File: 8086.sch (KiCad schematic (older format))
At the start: 1 part

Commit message: sfds
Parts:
- removed U?: 8086_Max_Mode, Package_DIP:DIP-40_W15.24mm, symbol MCU_Intel:8086_Max_Mode
- added U?: 8086_Min_Mode, Package_DIP:DIP-40_W15.24mm, symbol MCU_Intel:8086_Min_Mode
- added U? (x3): 74LS373, symbol 74xx:74LS373
- added U?: 74LS244, symbol 74xx:74LS244
- added U? (x2): 74LS245, symbol 74xx:74LS245
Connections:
- net labels added: GND, VCC
- wire segments 0 -> 124

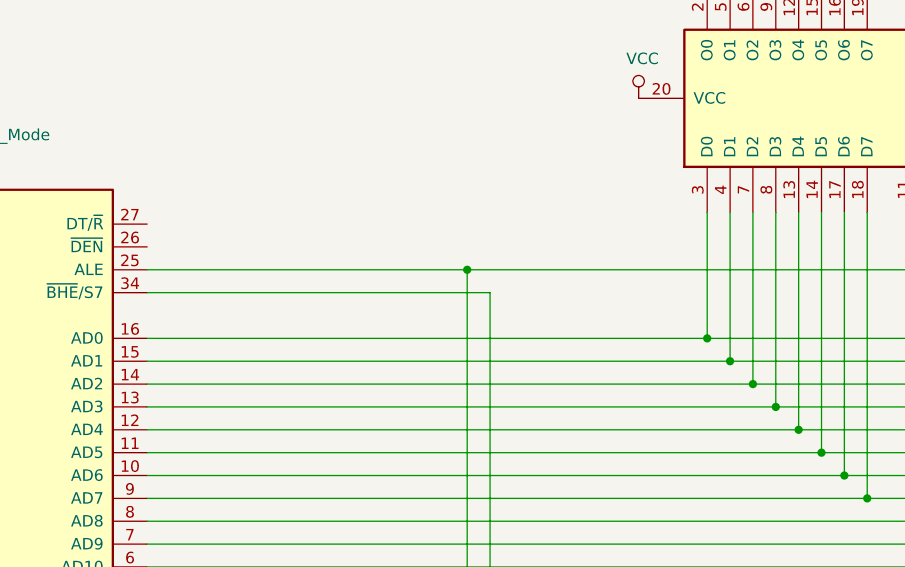
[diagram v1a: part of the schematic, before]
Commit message: 16550 v1
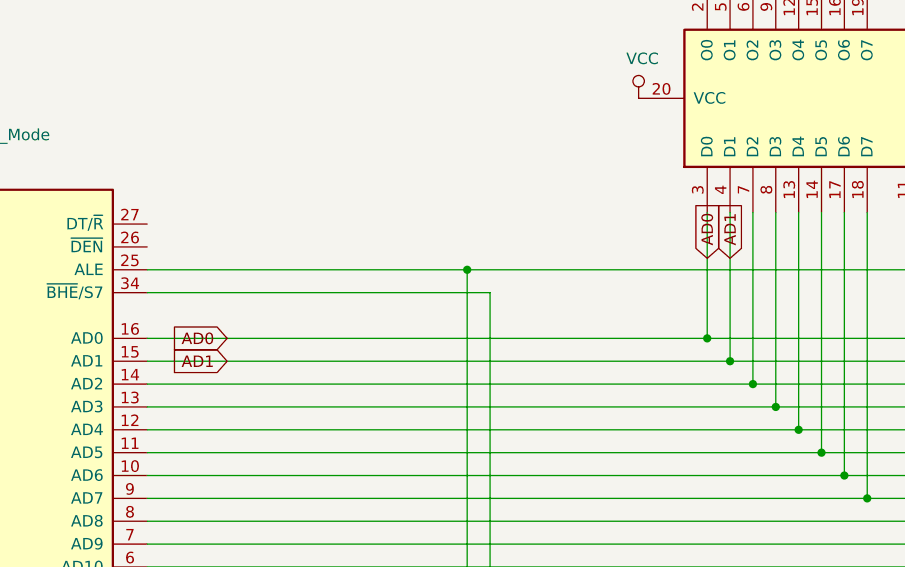
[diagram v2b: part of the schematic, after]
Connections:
- net labels added: AD0, AD1
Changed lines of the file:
@@
 $Descr A4 11693 8268
 encoding utf-8
-Sheet 3 5
+Sheet 3 7
 Title ""
 Date ""
@@
 	0    -1   -1   0
 $EndComp
-Wire Wire Line
-	5300 2850 8700 2850
 $Comp
 L power:GND #PWR?
@@
 	8900 3050 8900 2800
 Wire Wire Line
-	8800 2950 8800 2700
-Wire Wire Line
 	8700 2850 8700 2600
 Wire Wire Line
@@
 Connection ~ 5600 3150
 Connection ~ 5700 3250
-Connection ~ 5300 2850
 Connection ~ 5800 3350
 Wire Wire Line
 	5300 2300 5300 2850
-Wire Wire Line
-	5400 2300 5400 2950
 Wire Wire Line
 	5500 2300 5500 3050
@@
 	1    0    0    -1
 $EndComp
+Text GLabel 3200 2850 0    50   Input ~ 0
+AD0
+Text GLabel 3200 2950 0    50   Input ~ 0
+AD1
+Text GLabel 5400 2500 1    50   Input ~ 0
+AD1
+Text GLabel 5300 2500 1    50   Input ~ 0
+AD0
+Connection ~ 5300 2850
+Wire Wire Line
+	8800 2950 8800 2700
+Wire Wire Line
+	5400 2300 5400 2950
+Wire Wire Line
+	5300 2850 8700 2850
 $EndSCHEMATC

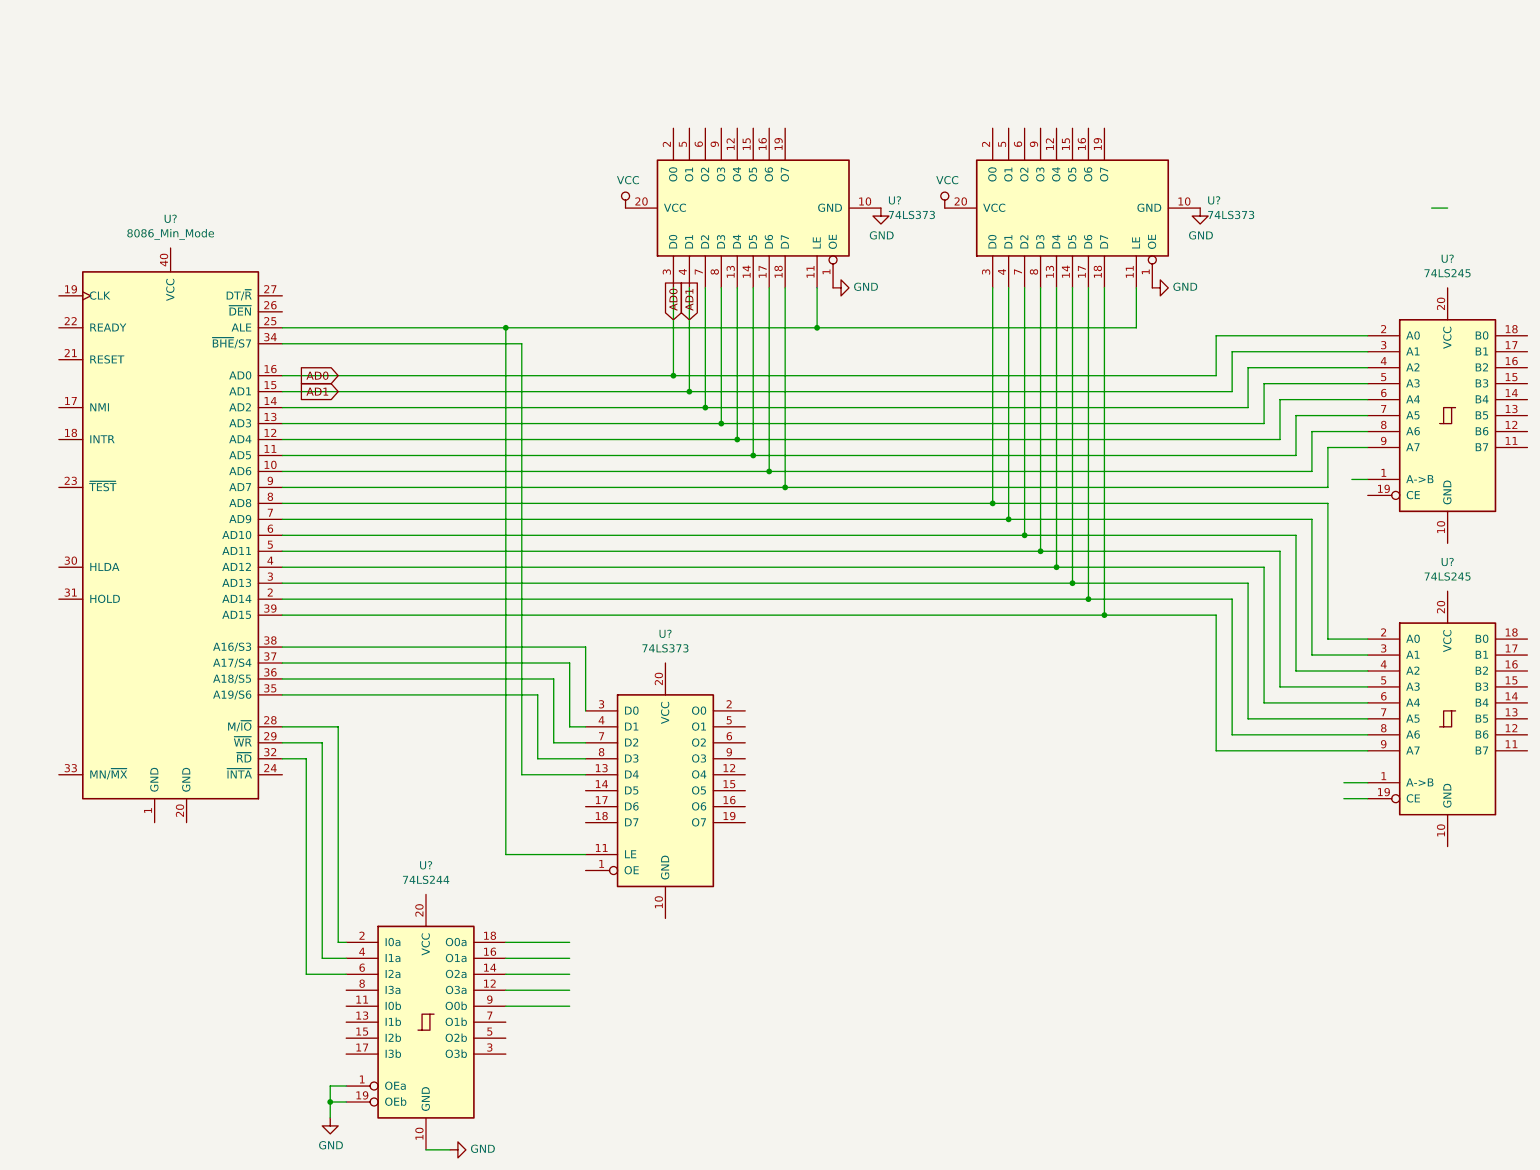
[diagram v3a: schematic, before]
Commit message: update
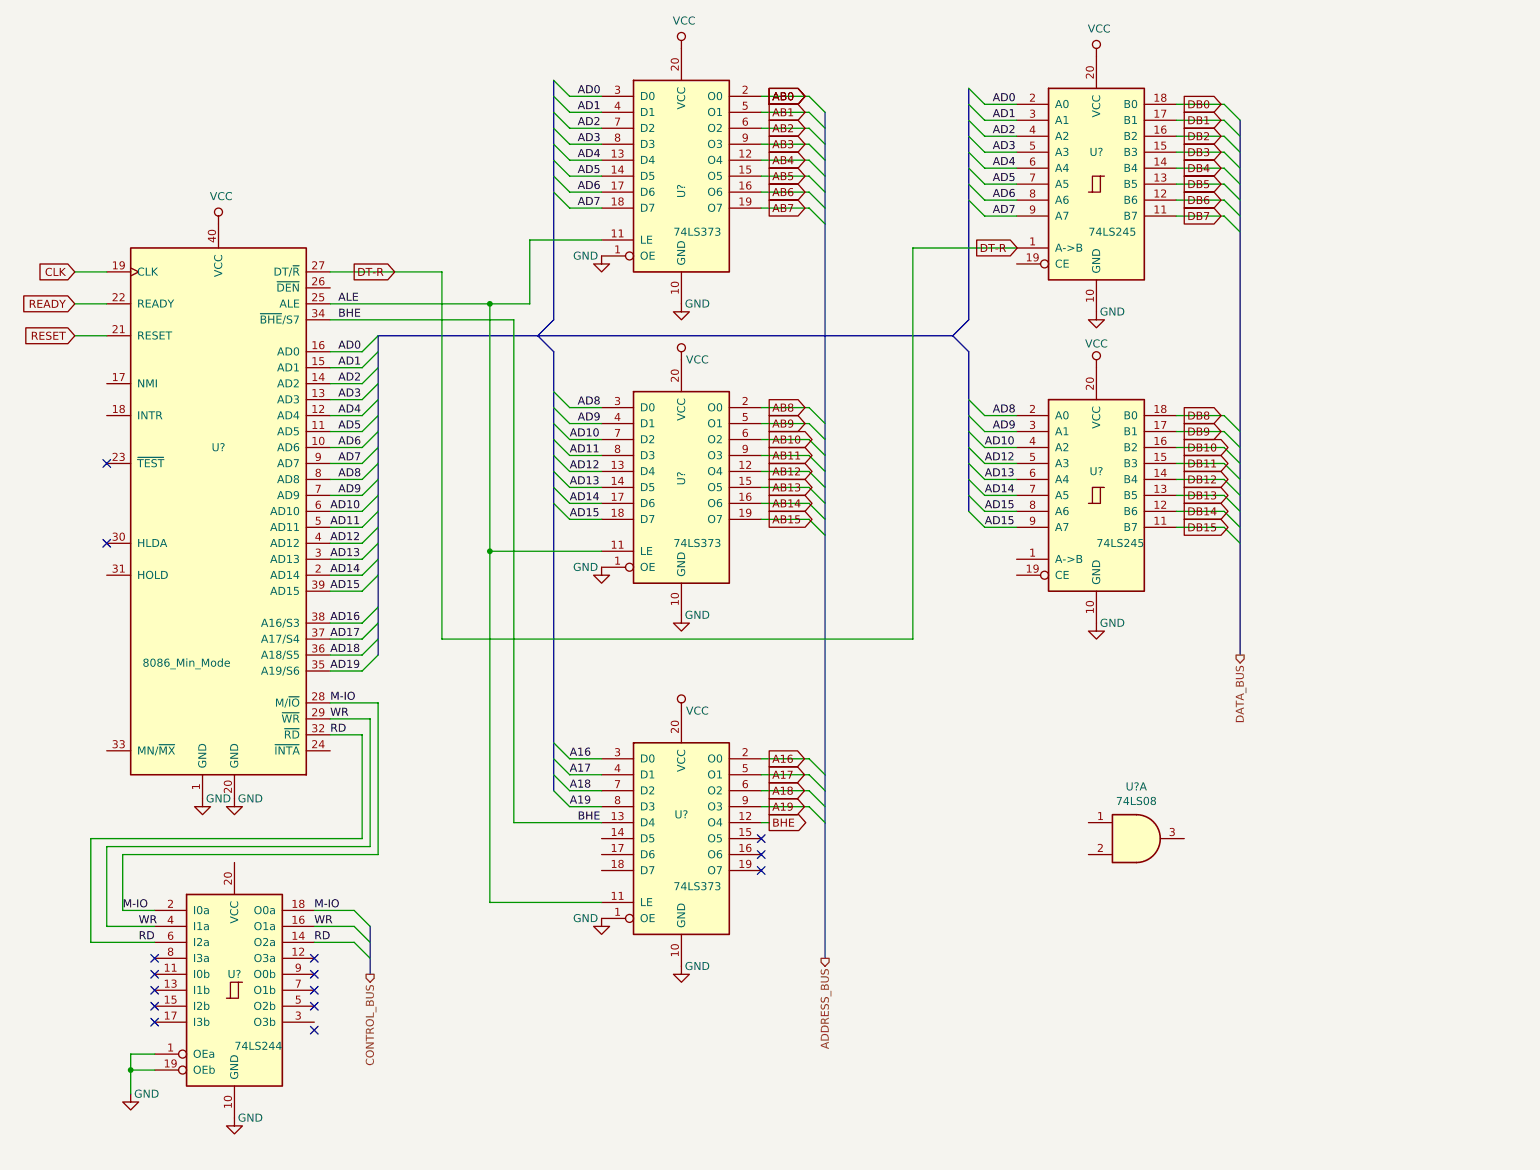
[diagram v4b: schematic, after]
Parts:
- removed U?: 8086_Min_Mode, Package_DIP:DIP-40_W15.24mm, symbol MCU_Intel:8086_Min_Mode
- removed U? (x3): 74LS373, symbol 74xx:74LS373
- removed U?: 74LS244, symbol 74xx:74LS244
- removed U? (x2): 74LS245, symbol 74xx:74LS245
- added U? (x2): 74LS245, symbol 74xx:74LS245
- added U?: 74LS244, symbol 74xx:74LS244
- added U? (x3): 74LS373, symbol 74xx:74LS373
- added U?: 74LS08, symbol 74xx:74LS08
- added U?: 8086_Min_Mode, Package_DIP:DIP-40_W15.24mm, symbol MCU_Intel:8086_Min_Mode
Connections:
- net labels added: A16, A17, A18, A19, AB0, AB1, AB10, AB11, AB12, AB13, AB14, AB15, AB2, AB3, AB4, AB5, AB6, AB7, AB8, AB9, AD10, AD11, AD12, AD13, AD14, AD15, AD16, AD17, AD18, AD19, AD2, AD3, AD4, AD5, AD6, AD7, AD8, AD9, ADDRESS_BUS, ALE, BHE, CLK, CONTROL_BUS, DATA_BUS, DB0, DB1, DB10, DB11, DB12, DB13, DB14, DB15, DB2, DB3, DB4, DB5, DB6, DB7, DB8, DB9, DT-R, M-IO, RD, READY, RESET, WR
- wire segments 124 -> 134
- no-connect marks 0 -> 15
